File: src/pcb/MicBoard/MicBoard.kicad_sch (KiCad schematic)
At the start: 1 part

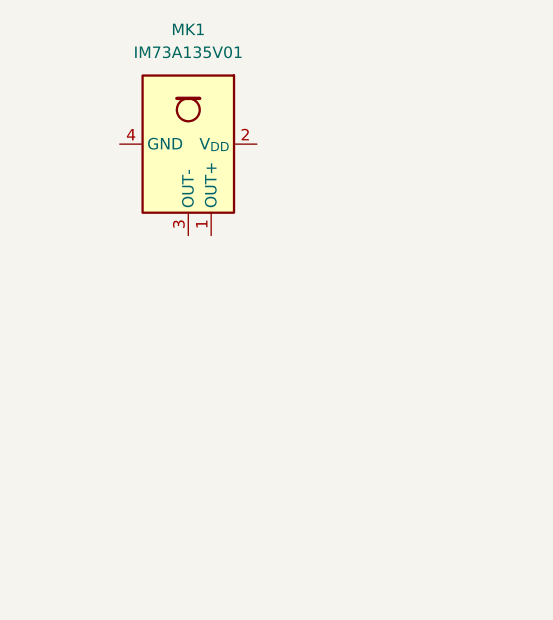
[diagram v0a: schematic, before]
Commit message: first schematic? maybe
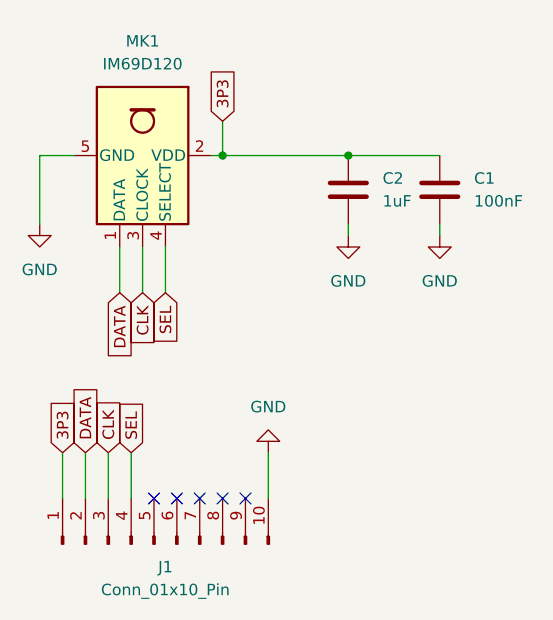
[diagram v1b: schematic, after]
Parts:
- removed MK1: IM73A135V01, Sensor_Audio:Infineon_PG-LLGA-5-2, symbol Sensor_Audio:IM73A135V01
- added C1: 100nF, symbol Device:C
- added C2: 1uF, symbol Device:C
- added J1: Conn_01x10_Pin, symbol Connector:Conn_01x10_Pin
- added MK1: IM69D120, Sensor_Audio:Infineon_PG-LLGA-5-1, symbol Sensor_Audio:IM69D120
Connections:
- new net 3P3: C1.1, C2.1, J1.1 (Pin_1), MK1.2 (VDD)
- new net CLK: J1.3 (Pin_3), MK1.3 (CLOCK)
- new net DATA: J1.2 (Pin_2), MK1.1 (DATA)
- new net GND: C1.2, C2.2, J1.10 (Pin_10), MK1.5 (GND)
- new net SEL: J1.4 (Pin_4), MK1.4 (SELECT)
- no-connect marks 0 -> 5
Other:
- company: (none) -> Armaan Gomes
- title: (none) -> Tiny Mic Board
